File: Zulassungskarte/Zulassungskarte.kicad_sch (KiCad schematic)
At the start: 28 parts, among them J1 Conn_02x04_Counter_Clockwise, J2 Conn_02x04_Counter_Clockwise, U1 ATmega48-20A

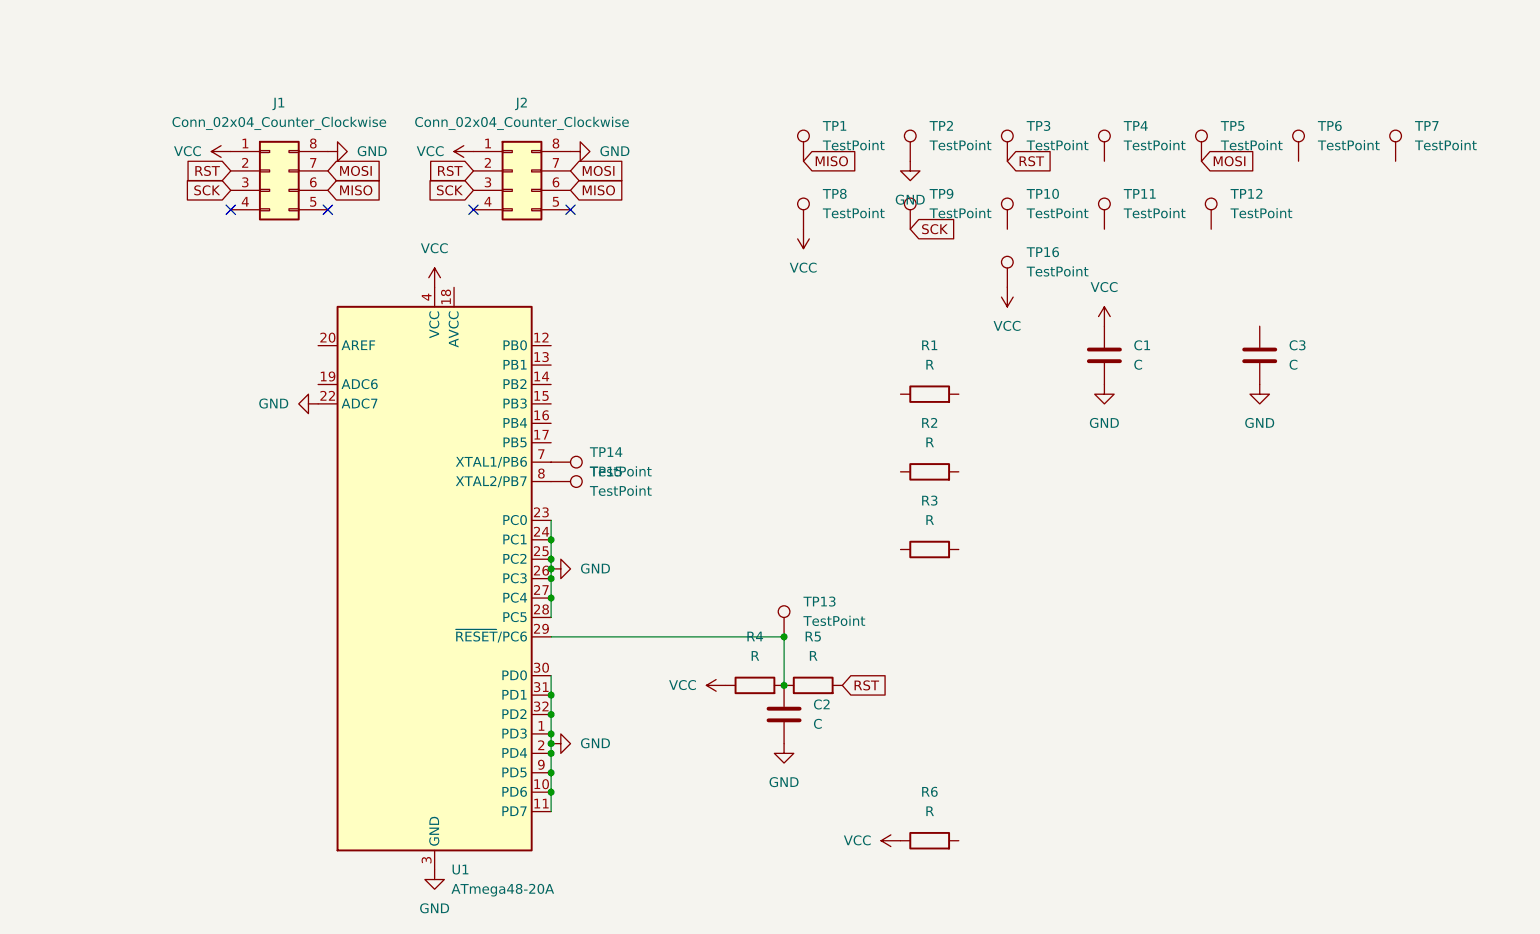
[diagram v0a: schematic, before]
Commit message: we
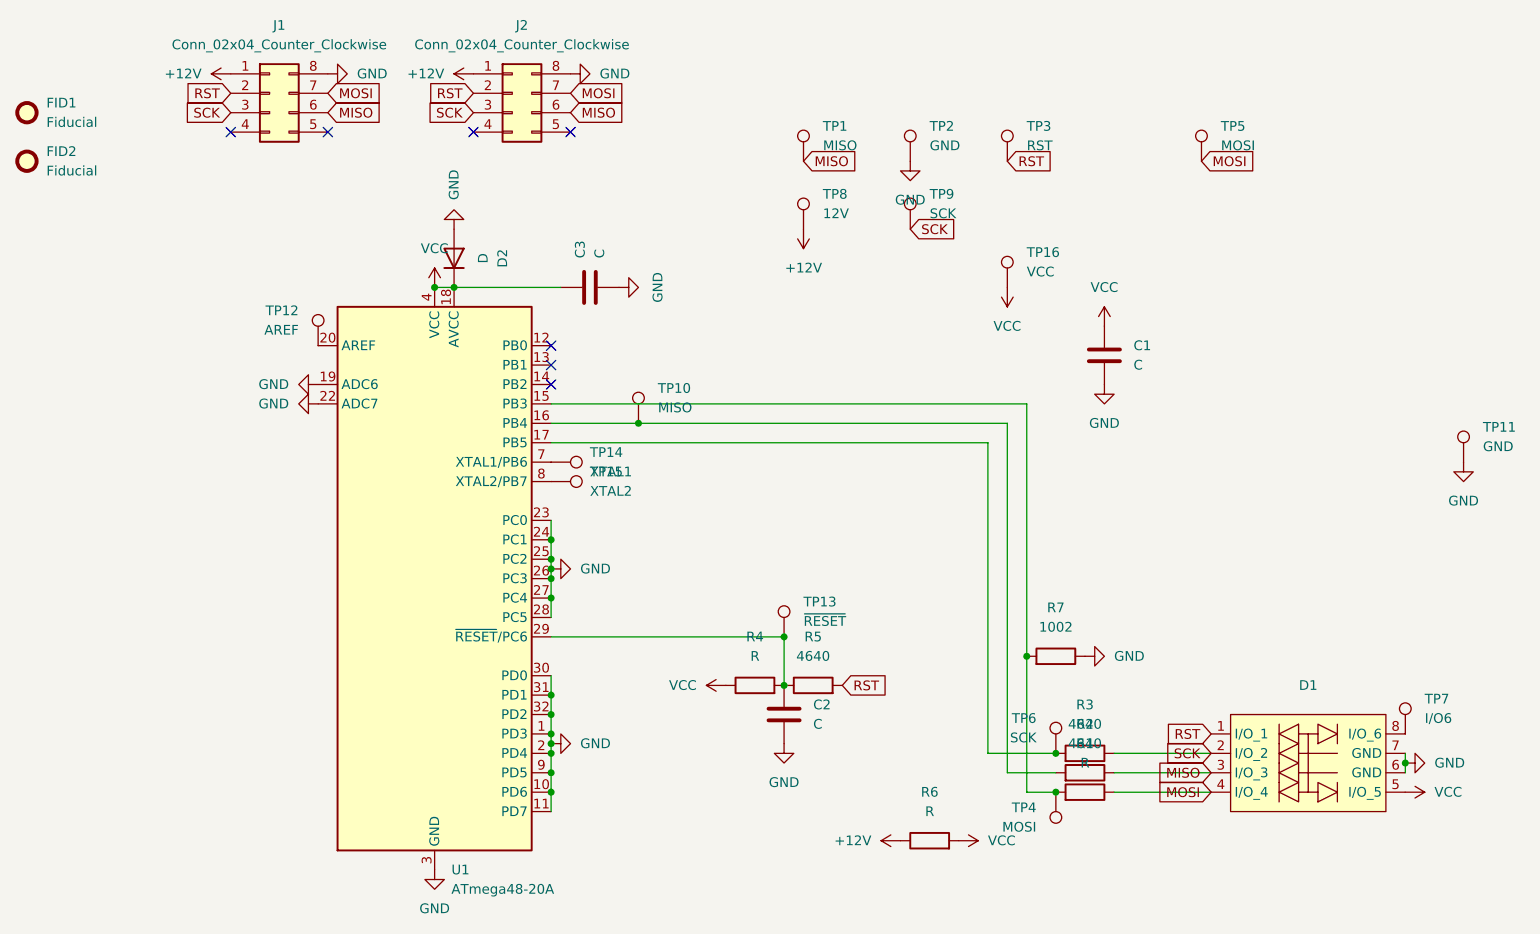
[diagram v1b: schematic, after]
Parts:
- added D1: ~, Package_SO:SO-8_3.9x4.9mm_P1.27mm, symbol Protection:ESDA6V1U1
- added D2: D, Diode_SMD:D_SOD-123, symbol Device:D
- added FID1, FID2: Fiducial, Fiducial:Fiducial_1.5mm_Mask3mm, symbol Mechanical:Fiducial
- added R7: 1002, Resistor_SMD:R_0805_2012Metric, symbol Device:R
- R2, R3, R5: value R -> 4640
- TP1, TP10: value TestPoint -> MISO
- TP11, TP2: value TestPoint -> GND
- TP12: value TestPoint -> AREF
- TP13: value TestPoint -> ~{RESET}
- TP14: value TestPoint -> XTAL1
- TP15: value TestPoint -> XTAL2
- TP16: value TestPoint -> VCC
- TP3: value TestPoint -> RST
- TP4, TP5: value TestPoint -> MOSI
- TP6, TP9: value TestPoint -> SCK
- TP7: value TestPoint -> I/O6
- TP8: value TestPoint -> 12V
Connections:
- net GND: now also TP11.1, U1.19 (ADC6), D1.6 (GND), D1.7 (GND), D2.2 (A), R7.1
- net MISO: now also R2.1, D1.3 (I/O_3)
- net MOSI: now also R1.1, D1.4 (I/O_4)
- net RST: now also D1.1 (I/O_1)
- net SCK: now also R3.1, D1.2 (I/O_2)
- net VCC: now also C3.1, R6.2, U1.18 (AVCC), D1.5 (I/O_5), D2.1 (K); no longer J1.1 (Pin_1), J2.1 (Pin_1), R6.1, TP8.1
- net at R1.2: now also TP4.1, U1.15 (PB3), R7.2
- net at TP12.1: now also U1.20 (AREF)
- net at TP10.1: now also R2.2, U1.16 (PB4)
- net at R3.2: now also TP6.1, U1.17 (PB5)
- net at TP7.1: now also D1.8 (I/O_6)
- new net +12V: J1.1 (Pin_1), J2.1 (Pin_1), R6.1, TP8.1
- no-connect marks 4 -> 7
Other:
- moved on the sheet: C3, J1, J2, R1, R2, R3, TP10, TP11, TP12, TP4, TP6, TP7
